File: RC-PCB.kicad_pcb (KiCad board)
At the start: 2 copper layers, 30 x 65 mm, 32 parts

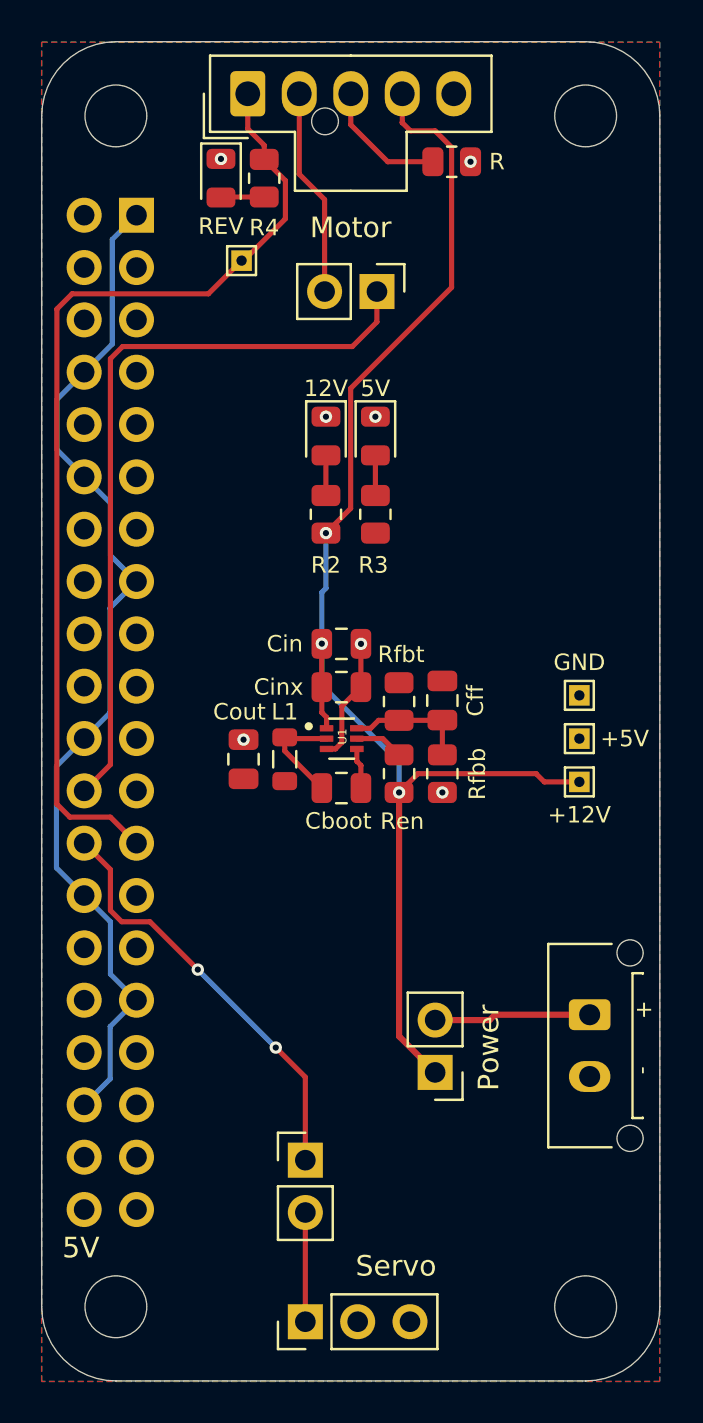
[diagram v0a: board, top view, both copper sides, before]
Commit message: ready to order
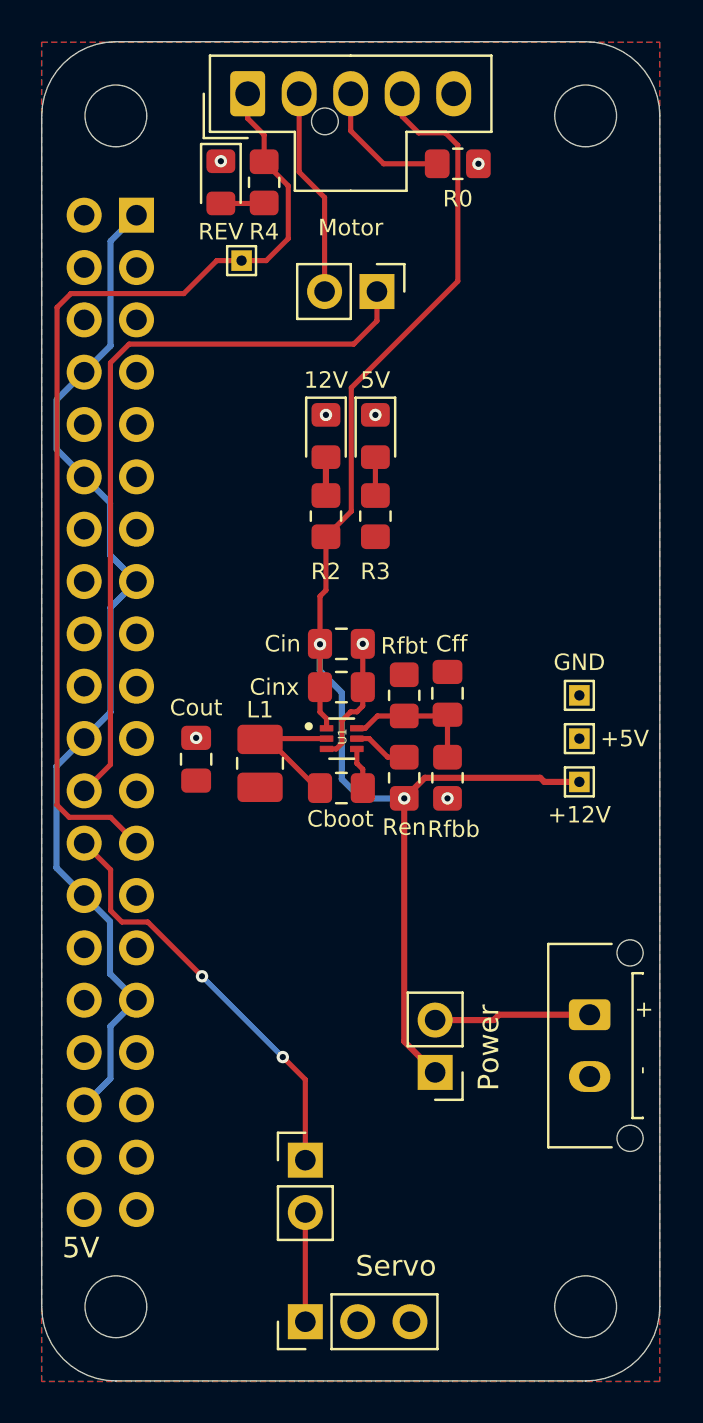
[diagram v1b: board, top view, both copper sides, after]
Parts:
- 12V, 5V: footprint LED_SMD:LED_0805_2012Metric -> LED_SMD:LED_0805_2012Metric_Pad1.15x1.40mm_HandSolder
- Cboot, Cff, Cin, Cinx, Cout: footprint Capacitor_SMD:C_0805_2012Metric -> Capacitor_SMD:C_0805_2012Metric_Pad1.18x1.45mm_HandSolder
- L1: footprint Inductor_SMD:L_0805_2012Metric -> Inductor_SMD:L_1008_2520Metric_Pad1.43x2.20mm_HandSolder
- R0: renamed from R; footprint Resistor_SMD:R_0805_2012Metric -> Resistor_SMD:R_0805_2012Metric_Pad1.20x1.40mm_HandSolder
- R2, R3, Ren, Rfbb, Rfbt: footprint Resistor_SMD:R_0805_2012Metric -> Resistor_SMD:R_0805_2012Metric_Pad1.20x1.40mm_HandSolder
- R4: value 650 -> 620; footprint Resistor_SMD:R_0805_2012Metric -> Resistor_SMD:R_0805_2012Metric_Pad1.20x1.40mm_HandSolder
- REV1: renamed from REV; value LED -> REV; footprint LED_SMD:LED_0805_2012Metric -> LED_SMD:LED_0805_2012Metric_Pad1.15x1.40mm_HandSolder
- moved Cout 2.30 mm to (141.8, 108.1)
- moved L1 1.22 mm to (144.9, 108.3)
- moved Cff 0.43 mm to (154.0, 104.9)
- moved Rfbt 0.39 mm to (151.9, 105.0)
- moved Ren 0.32 mm to (151.9, 109.0)
- moved Rfbb 0.32 mm to (154.0, 109.0)
- moved R0 0.31 mm to (154.5, 79.2)
- moved R4 0.20 mm to (145.1, 80.1)
- moved REV1 0.20 mm to (143.0, 80.1)
- moved R2 0.09 mm to (148.1, 96.3)
- moved R3 0.09 mm to (150.5, 96.3)
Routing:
- net Net-(U1-SW): track 5.26 -> 7.14 mm
- net +12V: track 67.6 -> 68.9 mm, vias 3 -> 2
- net /Rev: track 48.4 -> 49.2 mm
- net Net-(U1-FB): track 6.00 -> 6.74 mm
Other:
- board text added: "R"
- board text added: "~"
